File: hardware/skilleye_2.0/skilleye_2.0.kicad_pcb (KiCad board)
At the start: 2 copper layers, 4 parts, among them J1 TP4056 Breakout, U1 XIAO-ESP32-C6-SMD, U2 GY-521

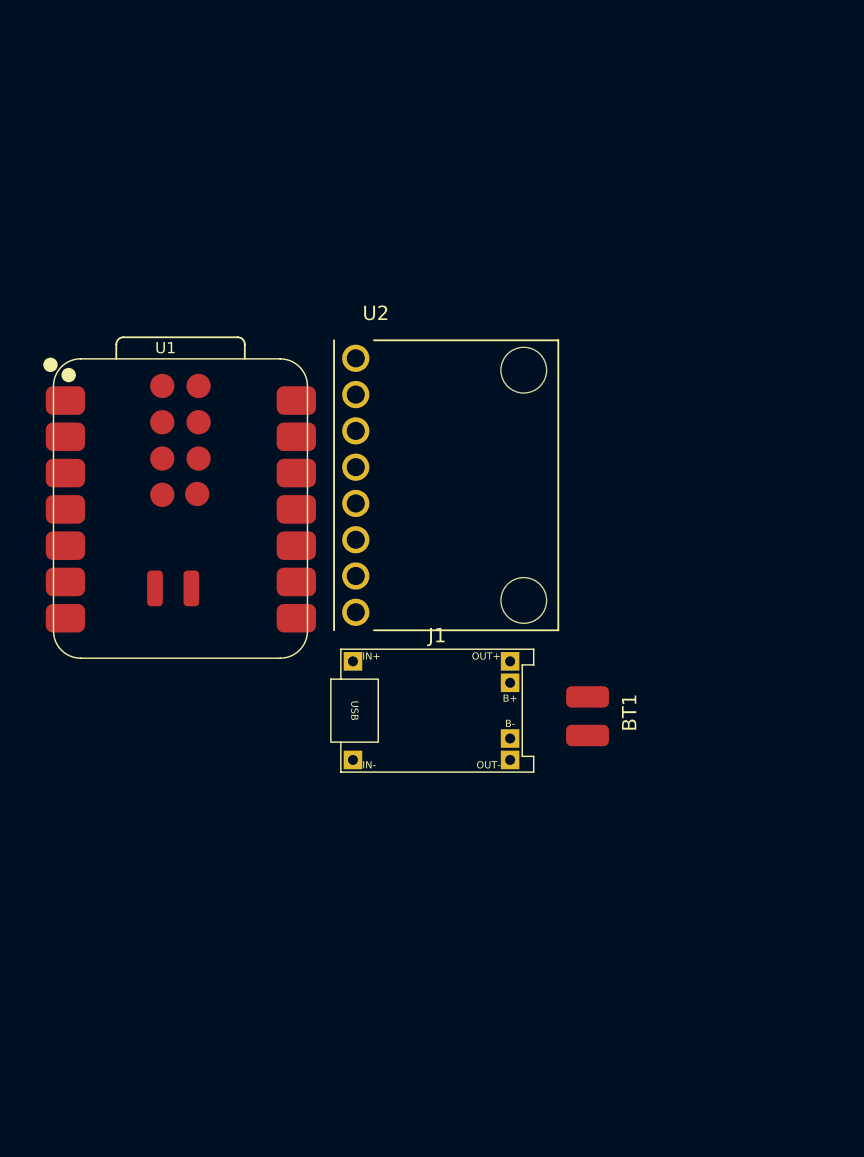
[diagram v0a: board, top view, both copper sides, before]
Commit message: added 2.0 pcb layout
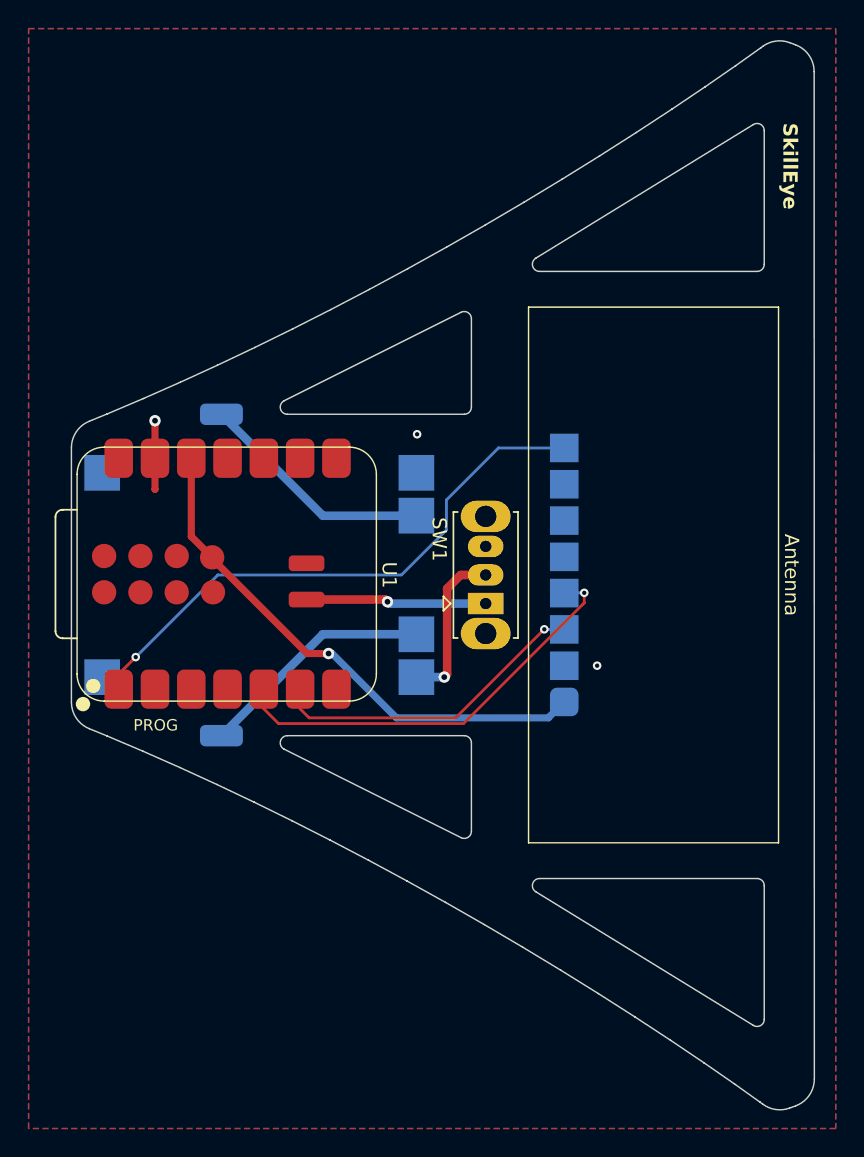
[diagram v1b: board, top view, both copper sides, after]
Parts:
- added G***: LOGO, LOGO, B.Cu at (156.0, 83.5)
- added SW1: SW_SPDT, Button_Switch_THT:SW_Slide_SPDT_Straight_CK_OS102011MS2Q, F.Cu at (144.0, 101.3)
- BT1, J1, U2: moved to B.Cu
- moved BT1 27.5 mm to (125.5, 99.3), turned to 90 degrees
- moved U1 22.9 mm to (136.4, 108.1), turned to 90 degrees
- moved U2 15.9 mm to (155.8, 99.3)
- moved J1 15.8 mm to (128.0, 99.3)
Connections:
- net Net-(BT1-+) renamed /BATT+
- net Net-(BT1--) renamed /BATT-
- J1 pad 5: Net-(J1-OUT+) -> /VBAT_RAW
- U1 pad 1: unconnected-(U1-D0-Pad1) -> /IMU_INT
- U1 pad 23: Net-(J1-OUT+) -> /VBAT_SW
- U2 pad INT: unconnected-(U2-PadINT) -> /IMU_INT
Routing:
- net /IMU_INT: track 0.00 -> 40.0 mm, vias 0 -> 1
- net +3V3: track 0.00 -> 37.4 mm, vias 0 -> 1
- net /SDA: track 0.00 -> 30.0 mm, vias 0 -> 1
- net /SCL: track 0.00 -> 22.7 mm, vias 0 -> 1
- net /BATT+: track 0.00 -> 16.6 mm
- net /BATT-: track 0.00 -> 16.6 mm
- net /VBAT_SW: track 0.00 -> 12.7 mm, vias 0 -> 1
- net /VBAT_RAW: track 0.00 -> 11.3 mm, vias 0 -> 1
- net GND: track 0.00 -> 4.80 mm, vias 0 -> 3
- added copper zone on B.Cu, net GND
- added copper zone on F.Cu, net GND
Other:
- board outline added: 52 x 74.8 mm
- board text added: "Antenna"
- board text added: "B+"
- board text added: "B-"
- board text added: "CHARGE"
- board text added: "PROG"
- board text added: "SkillEye"
- board text added: "TEAM: Purit • Rizal • Rachel • Jeslin • YuChing"
- board text added: "https://github.com/rizalfanex/SkillEye"
